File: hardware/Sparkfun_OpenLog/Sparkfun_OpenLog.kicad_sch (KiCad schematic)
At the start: 26 parts, among them Q1 16MHZ, U1 ATMEGA328P_TQFP, U2 3.3V MIC5205, U3 microSD Socket

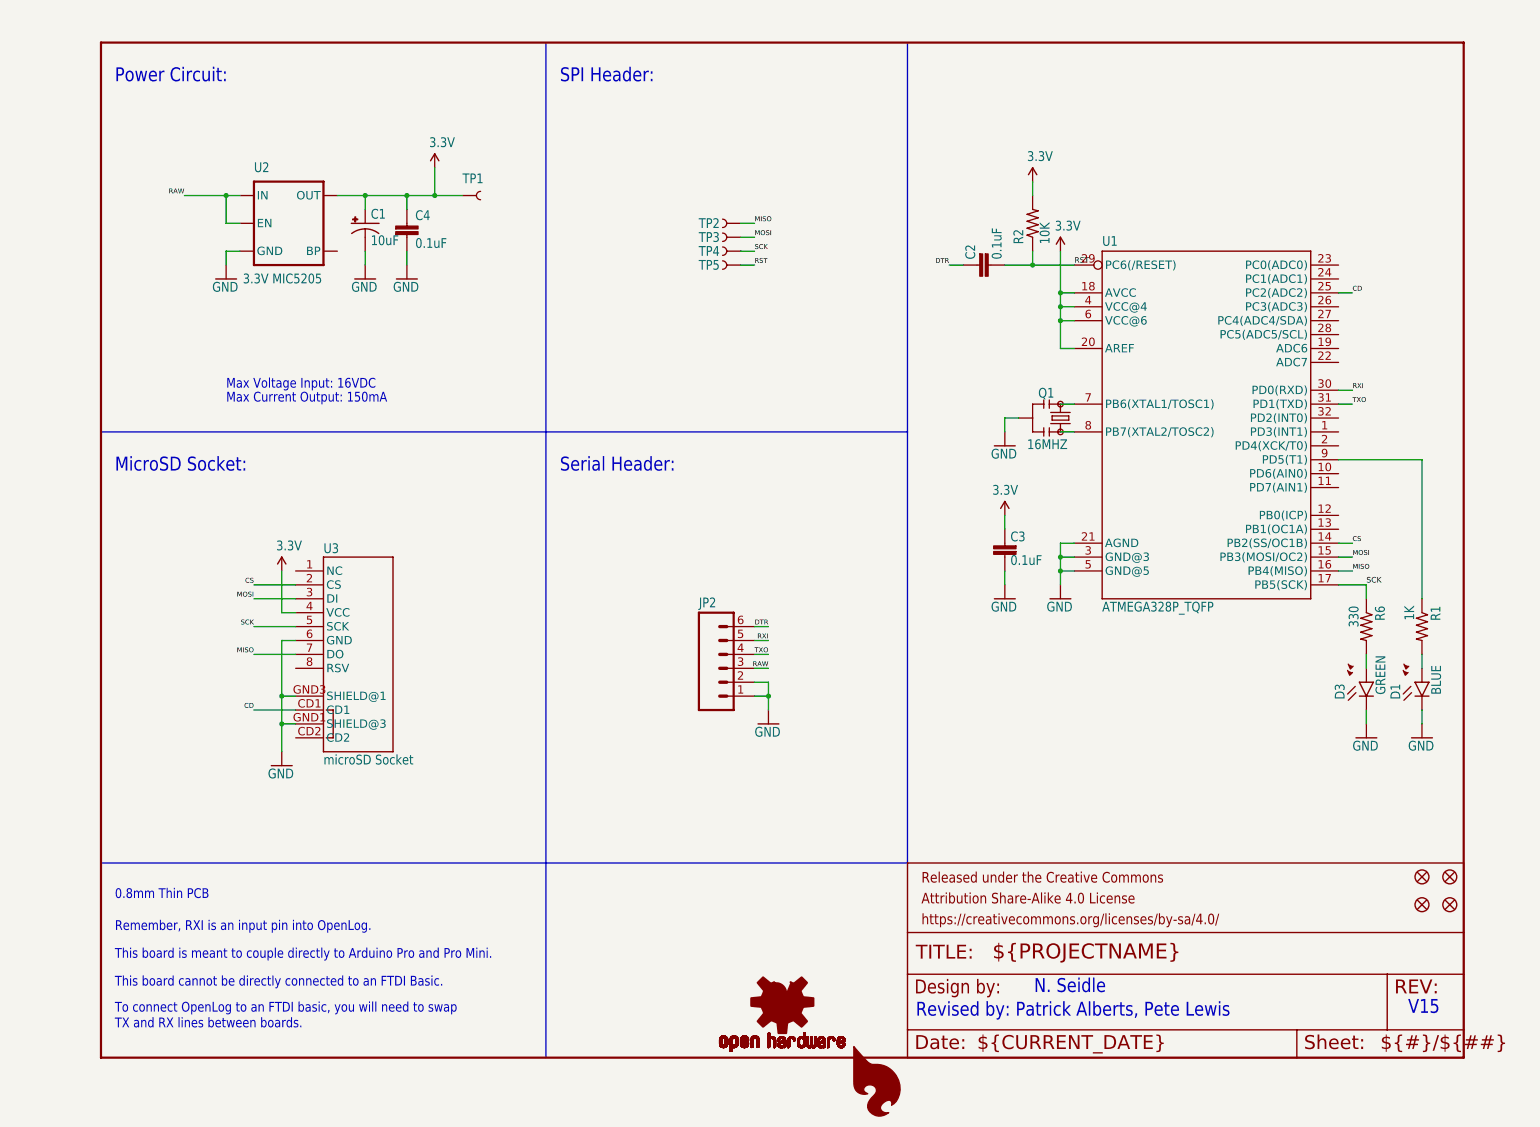
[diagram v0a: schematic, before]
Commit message: Updated Schematic
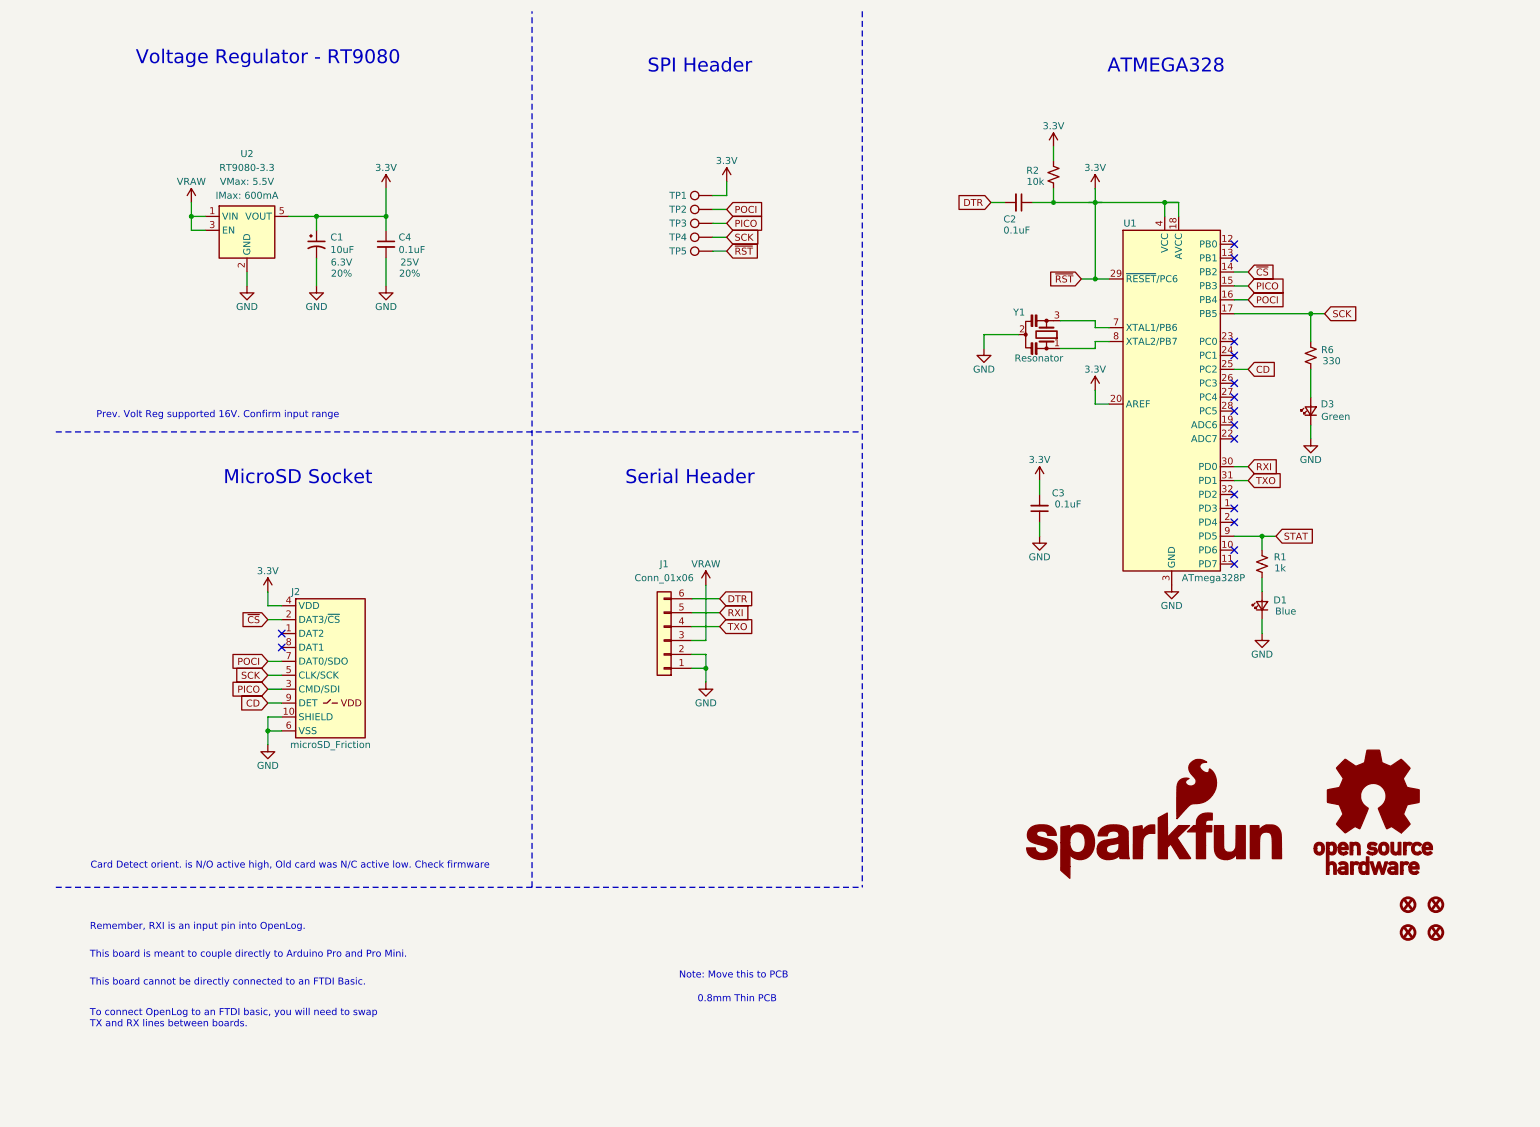
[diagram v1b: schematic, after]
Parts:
- removed FRAME1: FRAME-LETTER, Sparkfun_OpenLog:CREATIVE_COMMONS, symbol Sparkfun_OpenLog-eagle-import:FRAME-LETTER
- removed JP2: M06NO_SILK_FEMALE_PTH, Sparkfun_OpenLog:1X06_NO_SILK, symbol Sparkfun_OpenLog-eagle-import:M06NO_SILK_FEMALE_PTH
- removed LOGO1: SFE_LOGO_FLAME.1_INCH, Sparkfun_OpenLog:SFE_LOGO_FLAME_.1, symbol Sparkfun_OpenLog-eagle-import:SFE_LOGO_FLAME.1_INCH
- removed LOGO2: OSHW-LOGOMINI, Sparkfun_OpenLog:OSHW-LOGO-MINI, symbol Sparkfun_OpenLog-eagle-import:OSHW-LOGOMINI
- removed TP1, TP2, TP3, TP4, TP5: TEST-POINT3, Sparkfun_OpenLog:PAD.03X.03, symbol Sparkfun_OpenLog-eagle-import:TEST-POINT3
- removed U2: 3.3V MIC5205, Sparkfun_OpenLog:SOT23-5, symbol Sparkfun_OpenLog-eagle-import:MIC52053.3V
- removed U3: microSD Socket, Sparkfun_OpenLog:MICROSD_1_1, symbol Sparkfun_OpenLog-eagle-import:USD-SOCKET
- added G1: OSHW_Logo, SparkFun-Aesthetic:Creative_Commons_License, symbol SparkFun-Aesthetic:OSHW_Logo
- added G2: SparkFun_Logo, symbol SparkFun-Aesthetic:SparkFun_Logo
- added J1: Conn_01x06, SparkFun-Connector:1x06_P2.54mm, symbol SparkFun-Connector:Conn_01x06_P2.54mm
- added J2: microSD_Friction, SparkFun-Connector:microSD_Friction_Fit_Common, symbol SparkFun-Connector:microSD_Friction
- added TP1, TP2, TP3, TP4, TP5: 1.25mm, SparkFun-Connector:TestPoint-1.25mm, symbol SparkFun-Connector:TestPoint_1.25mm
- added U2: RT9080-3.3, SparkFun-Semiconductor-Standard:SOT23-5, symbol SparkFun-Regulator:RT9080-3.3
- C1: footprint Sparkfun_OpenLog:0603-POL -> SparkFun-Capacitor:C_0603_1608Metric_Polar; symbol Sparkfun_OpenLog-eagle-import:10UF-6.3V-20%(0603)(TANT){dblquote} -> SparkFun-Capacitor:10uF_0603_6.3V_20%_Polar(Tant); PROD_ID (none) -> CAP-13210; Tolerance (none) -> 20%; Voltage (none) -> 6.3V
- C2, C3, C4: footprint Sparkfun_OpenLog:0603-CAP -> SparkFun-Capacitor:C_0603_1608Metric; symbol Sparkfun_OpenLog-eagle-import:0.1UF-25V(+80/-20%)(0603) -> SparkFun-Capacitor:0.1uF_0603_25V_20%; PROD_ID (none) -> CAP-00810; Tolerance (none) -> 20%; Voltage (none) -> 25V
- D1: value BLUE -> Blue; footprint Sparkfun_OpenLog:LED-0603 -> SparkFun-LED:LED_0603_1608Metric_Blue; symbol Sparkfun_OpenLog-eagle-import:LED-BLUE0603 -> SparkFun-LED:LED_Blue_0603; PROD_ID (none) -> DIO-08575
- D3: value GREEN -> Green; footprint Sparkfun_OpenLog:LED-0603 -> SparkFun-LED:LED_0603_1608Metric_Green; symbol Sparkfun_OpenLog-eagle-import:LED-GREEN0603 -> SparkFun-LED:LED_Green_0603; PROD_ID (none) -> DIO-00821
- FID1, FID2, FID3, FID4: value FIDUCIALUFIDUCIAL -> Fiducial_0.5mm; footprint Sparkfun_OpenLog:MICRO-FIDUCIAL -> SparkFun-Aesthetic:Fiducial_0.5mm_Mask1mm; symbol Sparkfun_OpenLog-eagle-import:FIDUCIALUFIDUCIAL -> SparkFun-Aesthetic:Fiducial_0.5mm
- R1: value 1K -> 1k; footprint Sparkfun_OpenLog:0603-RES -> SparkFun-Resistor:R_0603_1608Metric; symbol Sparkfun_OpenLog-eagle-import:1KOHM-1/10W-1%(0603) -> SparkFun-Resistor:1k_0603; PROD_ID (none) -> RES-07856
- R2: value 10K -> 10k; footprint Sparkfun_OpenLog:0603-RES -> SparkFun-Resistor:R_0603_1608Metric; symbol Sparkfun_OpenLog-eagle-import:10KOHM-1/10W-1%(0603)0603 -> SparkFun-Resistor:10k_0603; PROD_ID (none) -> RES-00824
- R6: footprint Sparkfun_OpenLog:0603-RES -> SparkFun-Resistor:R_0603_1608Metric; symbol Sparkfun_OpenLog-eagle-import:330OHM1/10W1%(0603) -> SparkFun-Resistor:330_0603; PROD_ID (none) -> RES-00818
- U1: value ATMEGA328P_TQFP -> ATmega328P; footprint Sparkfun_OpenLog:TQFP32-08 -> SparkFun-Semiconductor-Standard:TQFP-32_7x7mm_P0.8mm; symbol Sparkfun_OpenLog-eagle-import:ATMEGA328P_TQFP -> SparkFun-IC-Microcontroller:ATmega328P-AU; PROD_ID (none) -> IC-09069
- Y1: renamed from Q1; value 16MHZ -> Resonator; footprint Sparkfun_OpenLog:RESONATOR-SMD -> SparkFun-Clock:Resonator_SMD_3.2x1.3mm; symbol Sparkfun_OpenLog-eagle-import:RESONATOR16MHZ -> SparkFun-Clock:Resonator_16MHz; PROD_ID (none) -> XTAL-08900
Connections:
- net RST is gone; now on net 3.3V: C2.1, R2.1, U1.29 (~{RESET}/PC6)
- net 3.3V: now also C1.1, J2.4 (VDD), TP1.1, TP5.1, U2.5 (VOUT); no longer C1.A (+)
- net CD: now also J2.9 (DET)
- net DTR: now also J1.6 (Pin_6)
- net GND: now also C1.2, D1.1 (K), D3.1 (K), J1.1 (Pin_1), J1.2 (Pin_2), J2.10 (SHIELD), J2.6 (VSS), U2.2 (GND); no longer C1.K (-), D1.C, D3.C
- net RXI: now also J1.5 (Pin_5)
- net SCK: now also J2.5 (CLK/SCK), TP4.1
- net TXO: now also J1.4 (Pin_4)
- net at R6.2: now also D3.2 (A); no longer D3.A
- net at R1.2: now also D1.2 (A); no longer D1.A
- net STAT: now reaches R1.1, U1.9 (PD5)
- net CS renamed ~{CS}
- net ~{CS}: now also J2.2 (DAT3/~{CS})
- net MISO renamed POCI
- net POCI: now also J2.7 (DAT0/SDO), TP2.1
- net MOSI renamed PICO
- net PICO: now also J2.3 (CMD/SDI), TP3.1
- new net VRAW: J1.3 (Pin_3), U2.1 (VIN), U2.3 (EN)
- no-connect marks 0 -> 16
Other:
- note added: "ATMEGA328"
- note added: "Card Detect orient. is N/O active high, Old card was N/C active low. Check firmware"
- note added: "MicroSD Socket"
- note added: "Note: Move this to PCB"
- note added: "Prev. Volt Reg supported 16V. Confirm input range"
- note added: "SPI Header"
- note added: "Serial Header"
- note added: "Voltage Regulator - RT9080"
- note removed: "Max Current Output: 150mA"
- note removed: "Max Voltage Input: 16VDC"
- note removed: "MicroSD Socket:"
- note removed: "N. Seidle"
- note removed: "Power Circuit:"
- note removed: "Revised by: Patrick Alberts, Pete Lewis"
- note removed: "SPI Header:"
- note removed: "Serial Header:"
- note removed: "V15"
- company: (none) -> Sparkfun Electronics
- title: (none) -> Sparkfun OpenLog

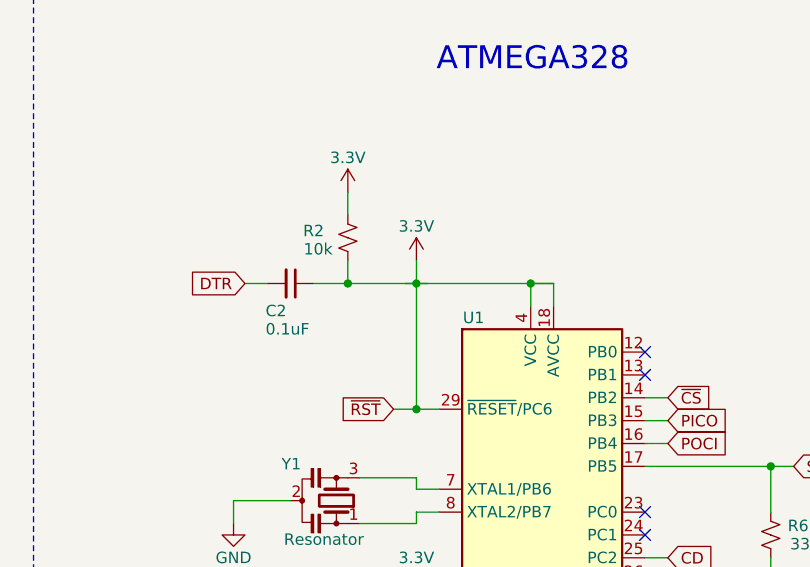
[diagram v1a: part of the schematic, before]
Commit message: Updated PCB File
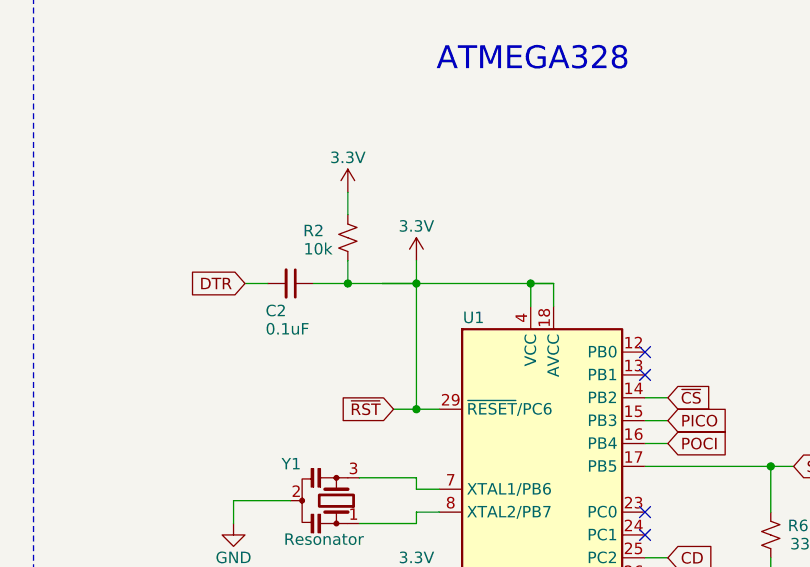
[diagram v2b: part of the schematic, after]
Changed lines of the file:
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@@
-	(wire
-		(pts
-			(xy 201.93 46.99) (xy 200.66 46.99)
-		)
-		(stroke
-			(width 0)
-			(type default)
-		)
-	)
 	(wire
 		(pts
@@
 			(width 0.1524)
 			(type solid)
+		)
+	)
+	(wire
+		(pts
+			(xy 198.12 46.99) (xy 201.93 46.99)
+		)
+		(stroke
+			(width 0)
+			(type default)
 		)
 	)
@@
 		)
 		(stroke
-			(width 0)
-			(type default)
-		)
-	)
-	(wire
-		(pts
-			(xy 201.93 46.99) (xy 203.2 46.99)
-		)
-		(stroke
